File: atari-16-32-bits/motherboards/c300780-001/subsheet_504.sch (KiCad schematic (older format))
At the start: 4 parts, among them Q500 LM78L82_TO92

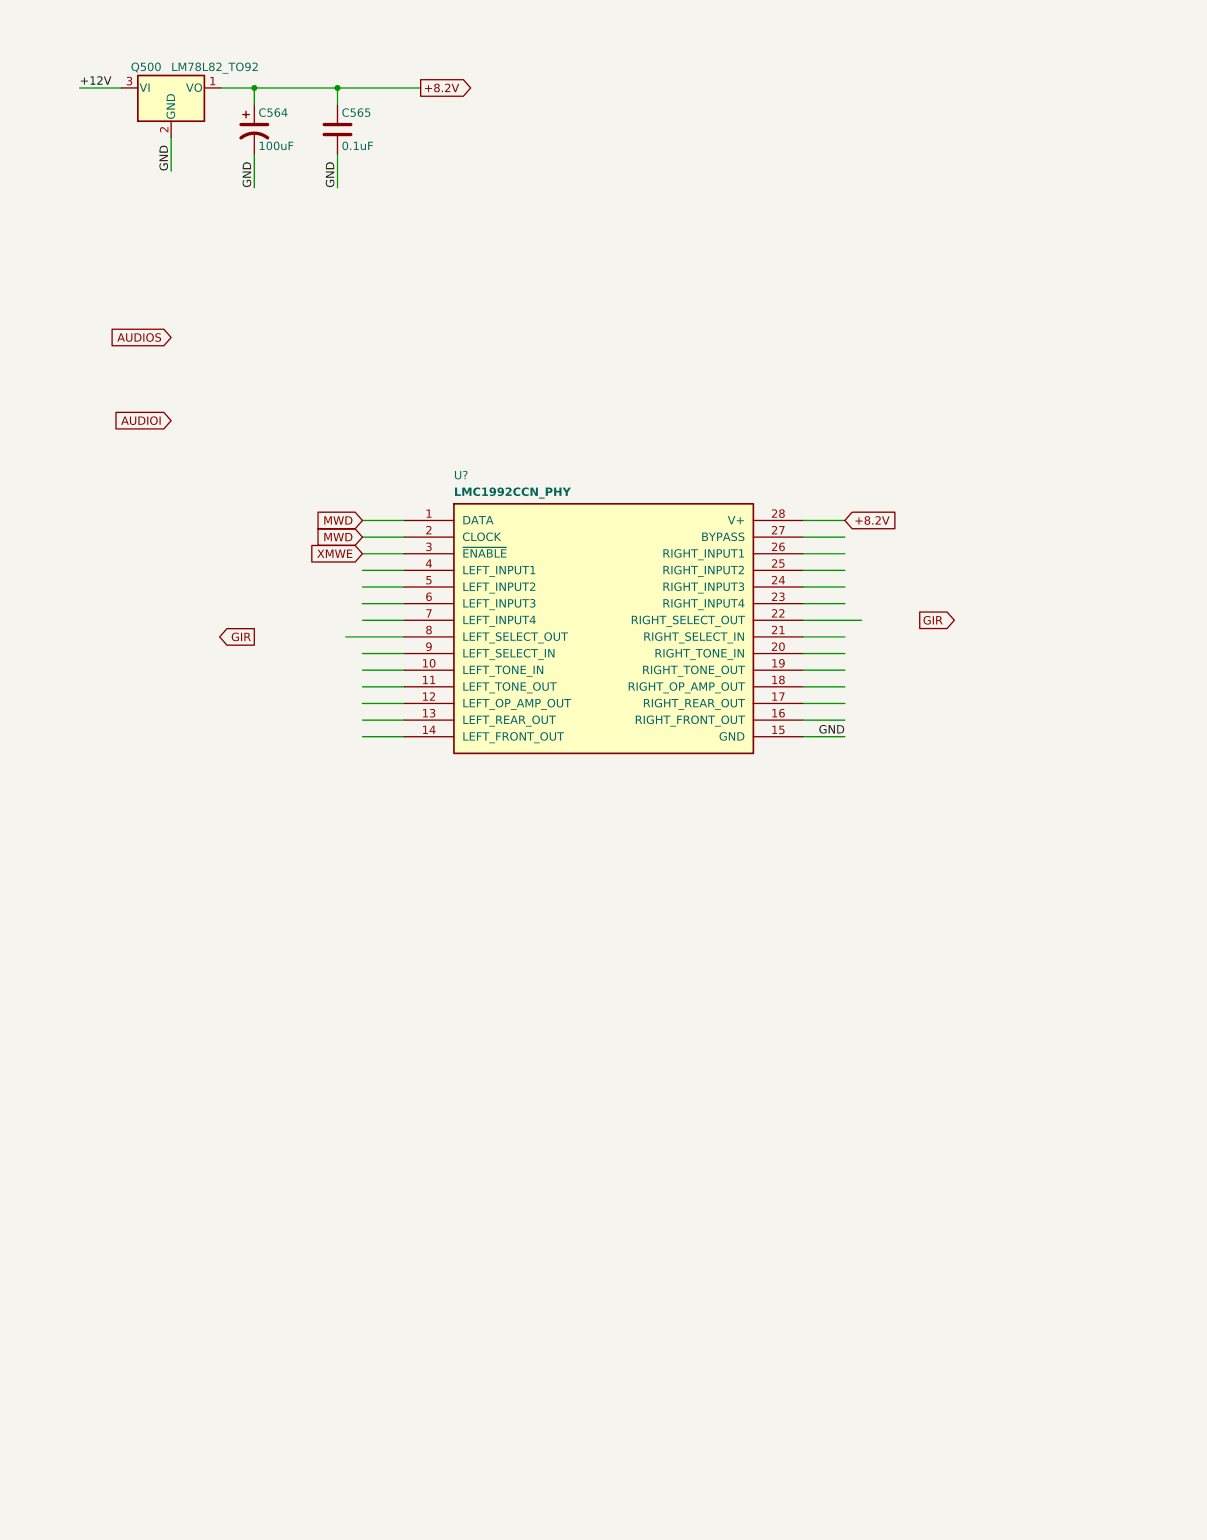
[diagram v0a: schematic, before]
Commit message: done subsheet 504 : audio mix
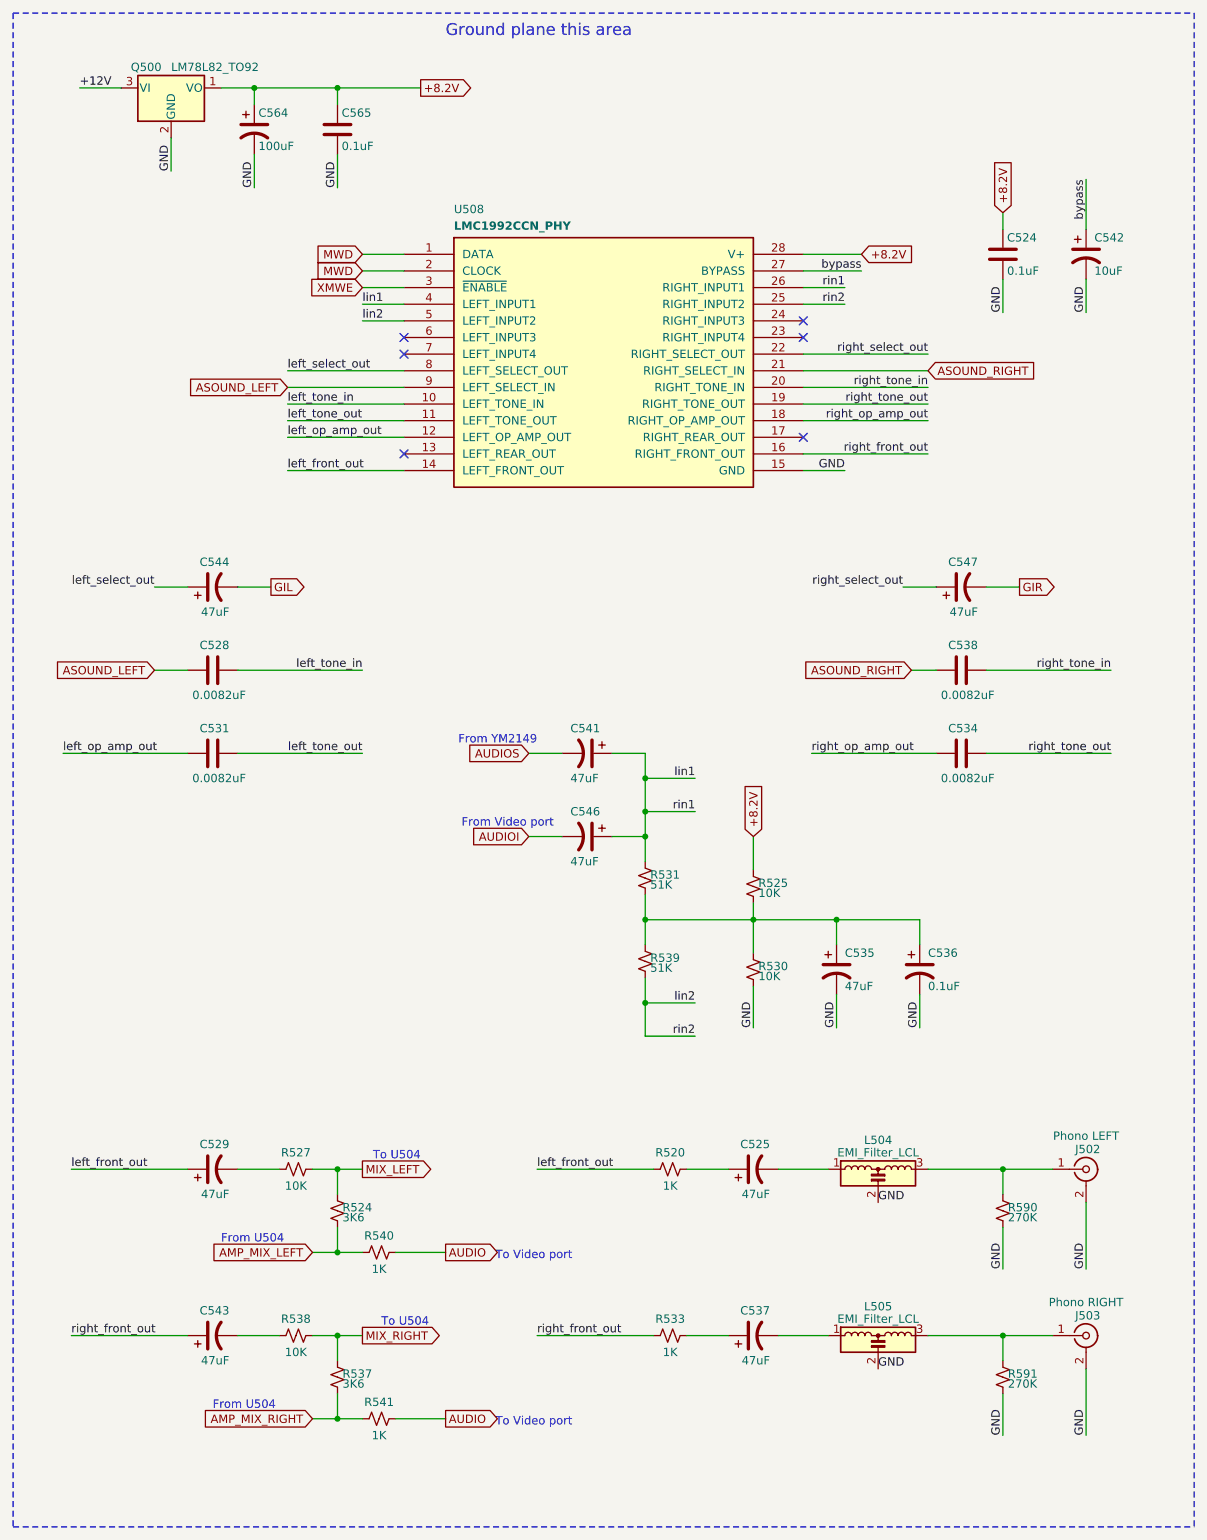
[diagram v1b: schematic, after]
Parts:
- added C524: 0.1uF, symbol Device:C
- added C525, C529, C535, C537, C541, C543, C544, C546, C547: 47uF, symbol Device:CP1
- added C528, C531, C534, C538: 0.0082uF, symbol Device:C
- added C536: 0.1uF, symbol Device:CP1
- added C542: 10uF, symbol Device:CP1
- added J502: Phono LEFT, symbol Connector:Conn_Coaxial
- added J503: Phono RIGHT, symbol Connector:Conn_Coaxial
- added L504, L505: EMI_Filter_LCL, symbol Device:EMI_Filter_LCL
- added R520, R533, R540, R541: 1K, symbol Device:R_Small_US
- added R524, R537: 3K6, symbol Device:R_Small_US
- added R525, R527, R530, R538: 10K, symbol Device:R_Small_US
- added R531, R539: 51K, symbol Device:R_Small_US
- added R590, R591: 270K, symbol Device:R_Small_US
- gave numbers to parts that had none: 1
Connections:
- net labels added: AMP_MIX_LEFT, AMP_MIX_RIGHT, ASOUND_LEFT, ASOUND_RIGHT, AUDIO, GIL, MIX_LEFT, MIX_RIGHT, bypass, left_front_out, left_op_amp_out, left_select_out, left_tone_in, left_tone_out, lin1, lin2, right_front_out, right_op_amp_out, right_select_out, right_tone_in, right_tone_out, rin1, rin2
- wire segments 37 -> 108
- no-connect marks 0 -> 6
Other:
- note added: "From U504"
- note added: "From Video port"
- note added: "From YM2149"
- note added: "Ground plane this area"
- note added: "To U504"
- note added: "To Video port"
- moved on the sheet: U508
